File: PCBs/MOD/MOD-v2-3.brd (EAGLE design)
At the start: 99.8 x 69.3 mm, 42 parts, among them J1 SERVO1, J10 JOY1, J11 JOY2, J12 RPi-Shutdown, J13 AN5, J14 AN6, J15 AN7, J16 AN8, J17 +5V (Main), J2 SERVO2, J3 TO Pi, J4 ACTUATORS, J5 +5V (Pi), J6 AN5, J7 AN6, J8 AN7, J9 AN8, SW2 500SSP1S2M2QEA, U1 ATTINY85

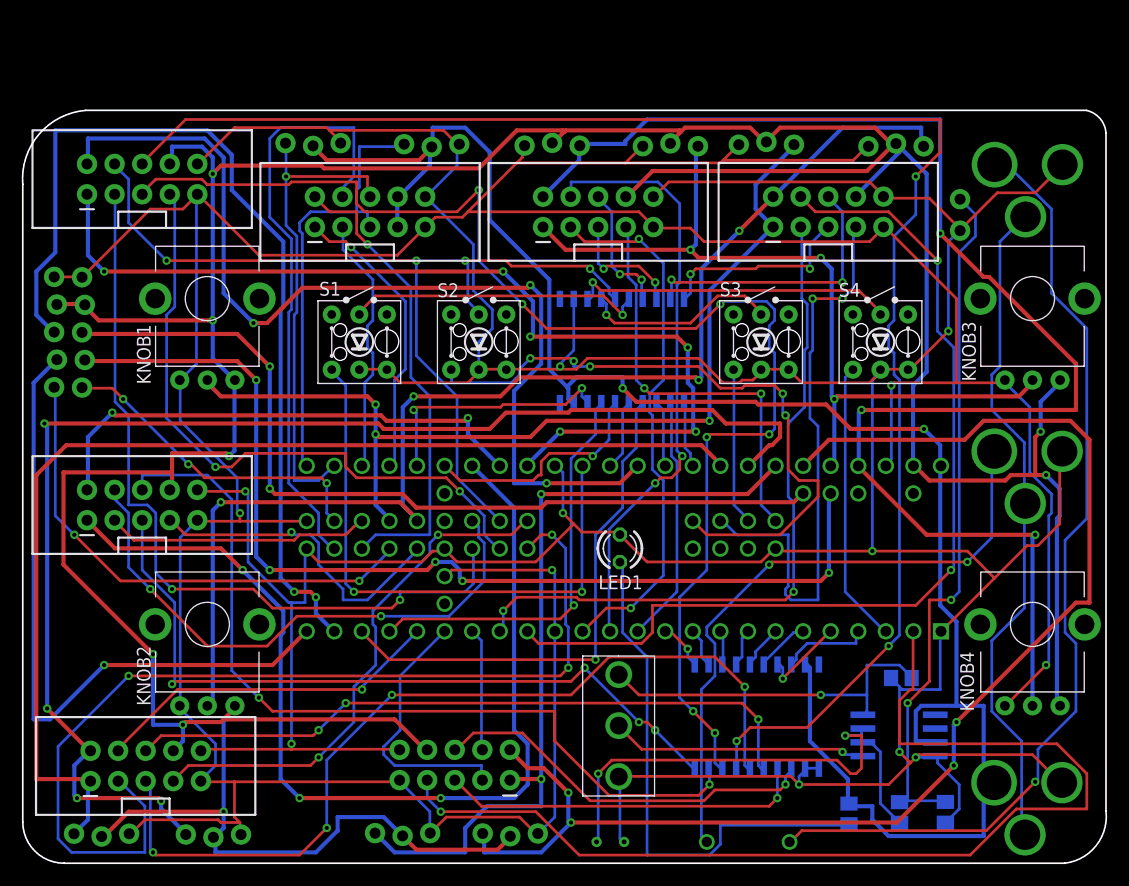
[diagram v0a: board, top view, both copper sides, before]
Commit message: tweaks to MOD pcb
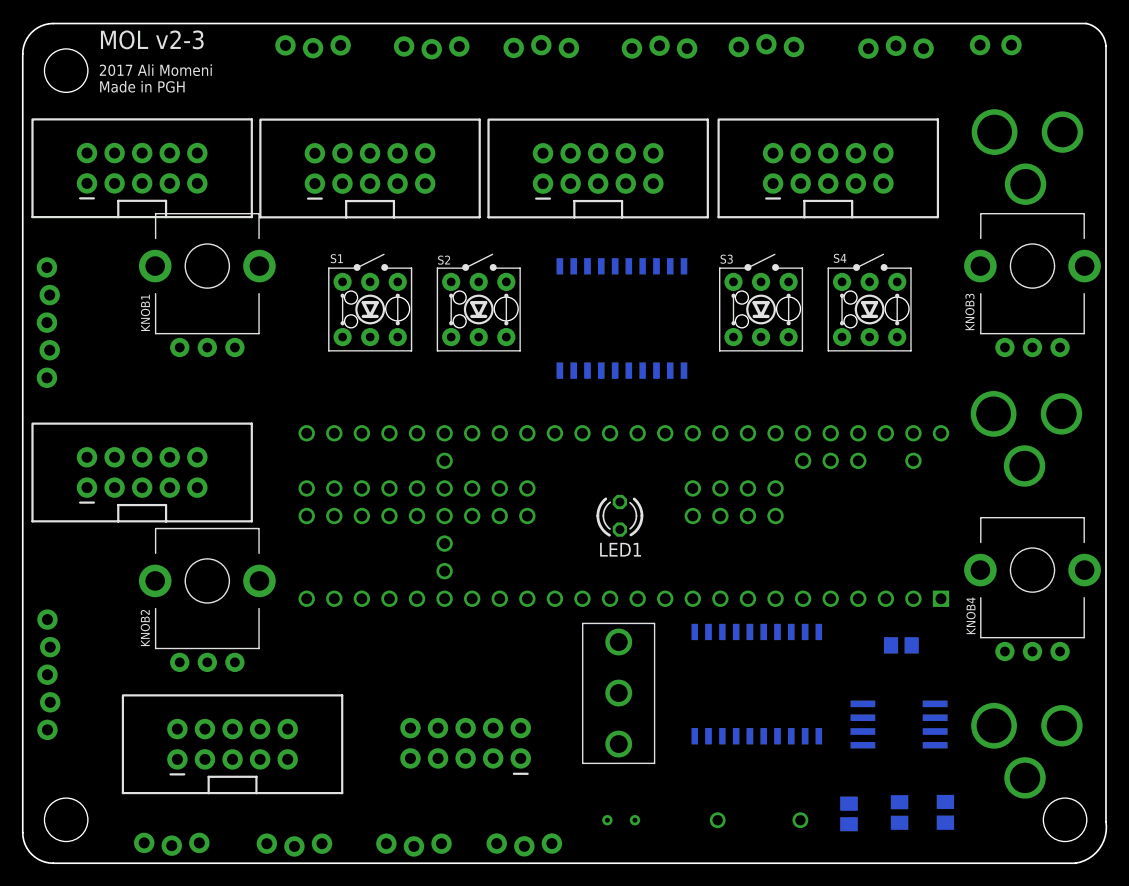
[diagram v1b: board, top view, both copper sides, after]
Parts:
- removed U$1: A2982, CMU-ArtFab:SOIC20
- added U2: A2982, CMU-ArtFab:SOIC20
- moved J11 31.6 mm to (2.40, 22.4)
- moved J12 14.5 mm to (88.3, 75.4), turned to 180 degrees
- moved J8 9.06 mm to (56.1, 75.2)
- moved J9 9.06 mm to (45.2, 75.2)
- moved J1 9.00 mm to (40.2, 75.1)
- moved J2 9.00 mm to (29.3, 75.2)
- moved J6 9.00 mm to (66.0, 75.3)
- moved J7 9.00 mm to (77.9, 75.2)
- moved STRIP3 8.25 mm to (19.3, 11.0)
- moved J14 7.51 mm to (27.6, 1.67)
- moved J13 6.52 mm to (16.3, 1.75)
- moved J17 5.24 mm to (103.1, 12.7)
- moved KNOB4 5.00 mm to (93.0, 27.0)
- moved J4 4.00 mm to (32.0, 64.0)
- moved KNOB2 4.00 mm to (17.0, 26.0)
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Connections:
- net +5V: now also U2.9; no longer U$1.9
- net GND: now also U2.11, U2.12; no longer U$1.11, U$1.12
- net PWM1: now also U2.8; no longer U$1.8
- net PWM2: now also U2.7; no longer U$1.7
- net PWM3: now also U2.6; no longer U$1.6
- net PWM4: now also U2.5; no longer U$1.5
- net PWM5: now also U2.4; no longer U$1.4
- net PWM6: now also U2.3; no longer U$1.3
- net PWM7: now also U2.2; no longer U$1.2
- net PWM8: now also U2.1; no longer U$1.1
- net PWM_1: now also U2.20; no longer U$1.20
- net PWM_2: now also U2.19; no longer U$1.19
- net PWM_3: now also U2.18; no longer U$1.18
- net PWM_4: now also U2.17; no longer U$1.17
- net PWM_5: now also U2.16; no longer U$1.16
- net PWM_6: now also U2.15; no longer U$1.15
- net PWM_7: now also U2.14; no longer U$1.14
- net PWM_8: now also U2.13; no longer U$1.13
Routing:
- net GND: track 422.0 -> 0.00 mm, vias 9 -> 0
- net AGND: track 363.0 -> 0.00 mm, vias 8 -> 0
- net +3V3: track 356.3 -> 0.00 mm, vias 4 -> 0
- net +5V: track 172.0 -> 0.00 mm, vias 2 -> 0
- net PWM_4: track 146.7 -> 0.00 mm, vias 3 -> 0
- net AN12: track 132.5 -> 0.00 mm, vias 3 -> 0
- net PWM_3: track 124.2 -> 0.00 mm, vias 7 -> 0
- net AN6: track 123.5 -> 0.00 mm, vias 4 -> 0
- net AN8: track 123.1 -> 0.00 mm, vias 4 -> 0
- net AN10: track 115.4 -> 0.00 mm, vias 4 -> 0
- net AN5: track 103.6 -> 0.00 mm
- net LED4: track 99.0 -> 0.00 mm, vias 1 -> 0
- net JOYV1: track 95.3 -> 0.00 mm, vias 5 -> 0
- net AN1: track 92.6 -> 0.00 mm, vias 3 -> 0
- net AN3: track 91.6 -> 0.00 mm, vias 6 -> 0
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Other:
- board size 99.8 x 69.3 mm -> 99.8 x 77.3 mm
